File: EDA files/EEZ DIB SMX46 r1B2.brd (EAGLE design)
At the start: 146 x 95 mm, 159 parts, among them IC1 STM32F030C6T6, IC2 74HC1G126GW,125, IC3 M24C32-WMN6P, IC4 LP2985-33DBVR, IC5 74HC2G04GW,125, IC6 OPA2990IDR, K1 FTR-C1GA012G-B05, K10 FTR-C1GA012G-B05, K11 FTR-C1GA012G-B05, K12 FTR-C1GA012G-B05, K13 FTR-C1GA012G-B05, K14 FTR-C1GA012G-B05, K15 FTR-C1GA012G-B05, K16 FTR-C1GA012G-B05, K17 FTR-C1GA012G-B05, K18 FTR-C1GA012G-B05, K19 FTR-C1GA012G-B05, K2 FTR-C1GA012G-B05, K20 FTR-C1GA012G-B05, K21 FTR-C1GA012G-B05, K22 FTR-C1GA012G-B05, K23 FTR-C1GA012G-B05, K24 FTR-C1GA012G-B05, K3 FTR-C1GA012G-B05, K4 FTR-C1GA012G-B05, K5 FTR-C1GA012G-B05, K6 FTR-C1GA012G-B05, K7 FTR-C1GA012G-B05, K8 FTR-C1GA012G-B05, K9 FTR-C1GA012G-B05, Q1 2N7002, Q10 2N7002, Q11 2N7002, Q12 2N7002, Q13 2N7002, Q14 2N7002, Q15 2N7002, Q16 2N7002, Q17 2N7002, Q18 2N7002, Q19 2N7002, Q2 2N7002, Q20 2N7002, Q21 2N7002, Q22 2N7002, Q23 2N7002, Q24 2N7002, Q25 2N7002, Q3 2N7002, Q4 2N7002, Q5 2N7002, Q6 2N7002, Q7 2N7002, Q8 2N7002, Q9 2N7002, X1 N.C., X2 77317-104-28LF, X3 691327310016, X4 691327310016

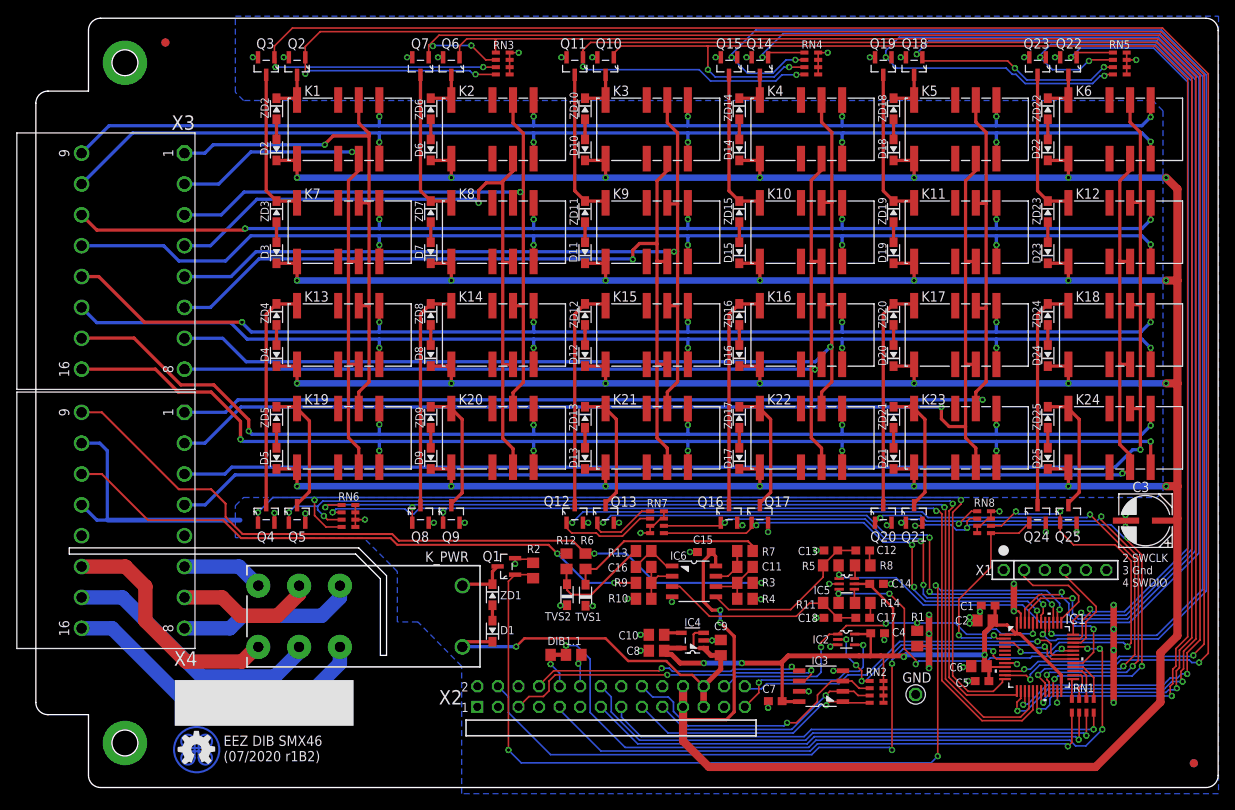
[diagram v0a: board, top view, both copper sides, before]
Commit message: Gerbers update
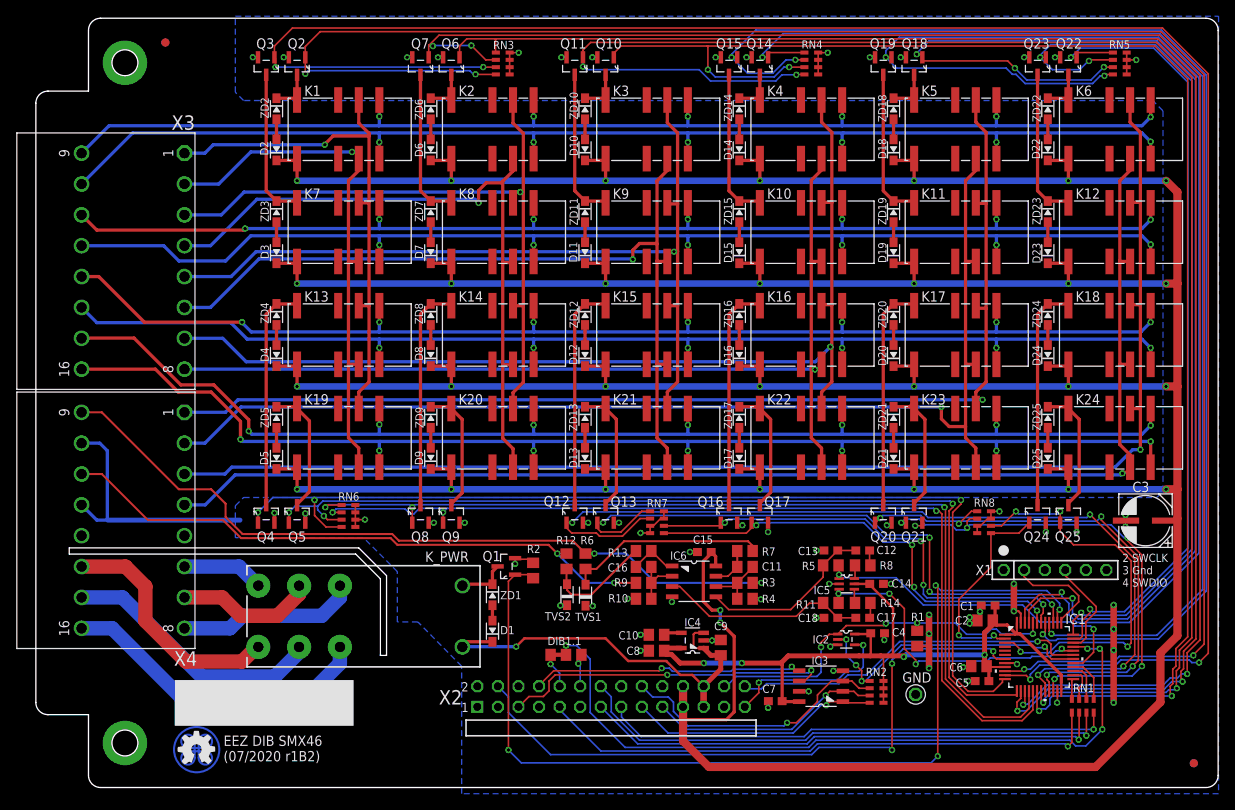
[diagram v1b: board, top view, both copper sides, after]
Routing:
- net +12V: track 723.7 -> 732.5 mm
